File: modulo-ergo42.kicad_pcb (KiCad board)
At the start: 2 copper layers, 135.9 x 79.4 mm, 38 parts, among them J1 AudioJack4_Ground, J2 AudioJack4_Ground, J3 AudioJack4_Ground, J4 AudioJack4_Ground, SW1 SW_Push, SW10 SW_Push, SW11 SW_Push, SW12 SW_Push, SW13 SW_Push, SW14 SW_Push, SW15 SW_Push, SW16 SW_Push, SW17 SW_Push, SW18 SW_Push, SW19 SW_Push, SW2 SW_Push, SW20 SW_Push, SW21 SW_Push, SW22 SW_Push, SW23 SW_Push, SW24 SW_Push, SW25 SW_Push, SW26 SW_Push, SW27 SW_Push, SW28 SW_Push, SW29 SW_DIP_x02, SW3 SW_Push, SW4 SW_Push, SW5 SW_Push, SW6 SW_Push, SW7 SW_Push, SW8 SW_Push, SW9 SW_Push, U1 TCA9555PWR, U2 TCA9555PWR

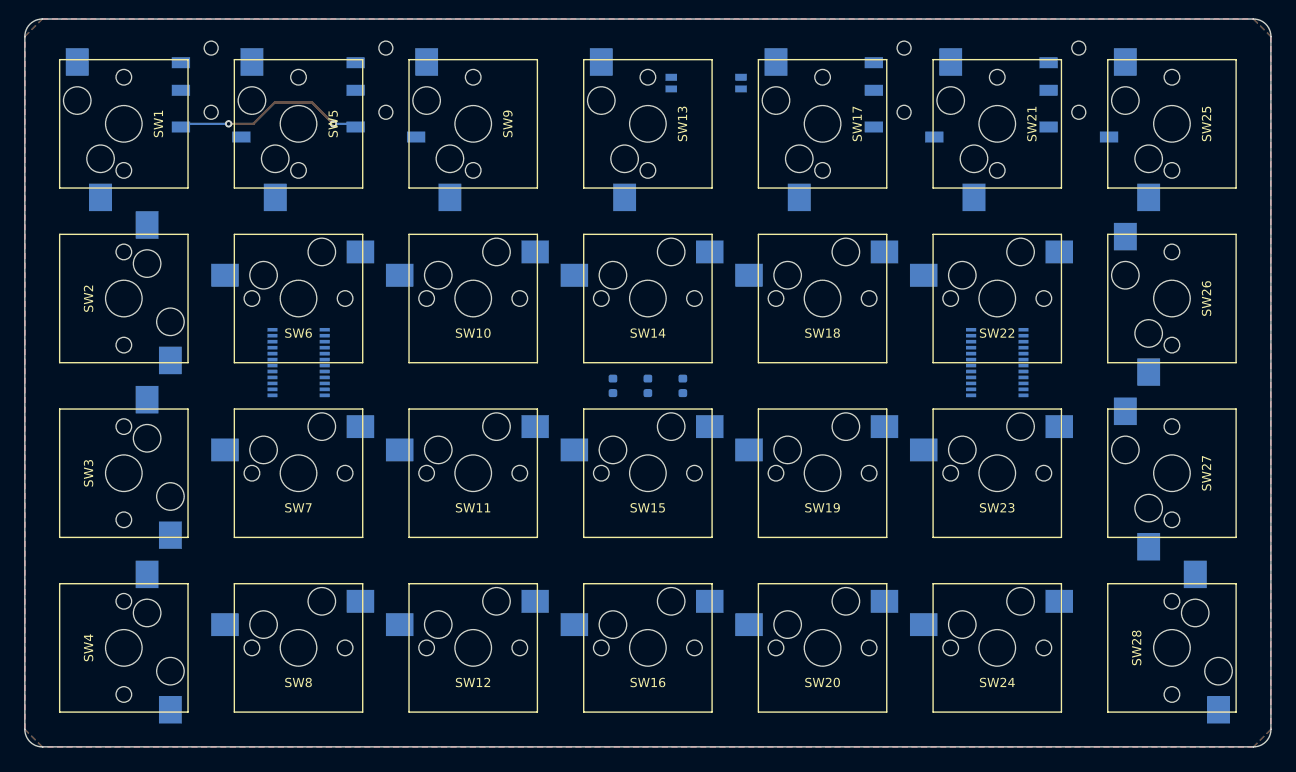
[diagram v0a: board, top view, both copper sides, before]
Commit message: Fix schematics
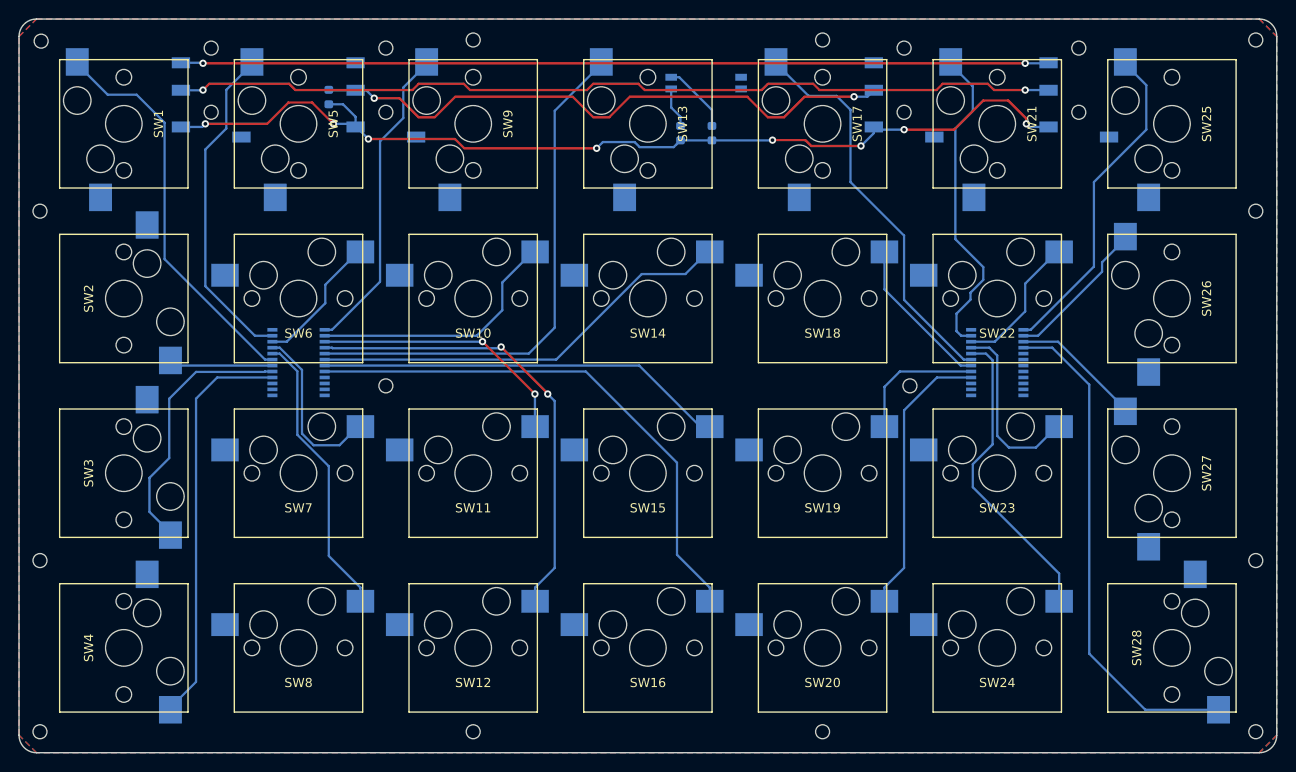
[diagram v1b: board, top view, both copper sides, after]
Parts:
- added ?: Screw_Hole, library:Screw_Hole, F.Cu at (56.9, 55.2)
- added ?: Screw_Hole, library:Screw_Hole, F.Cu at (142.2, 112.0)
- added ?: Screw_Hole, library:Screw_Hole, F.Cu at (189.5, 112.0)
- added ?: Screw_Hole, library:Screw_Hole, F.Cu at (189.5, 36.6)
- added ?: Screw_Hole, library:Screw_Hole, F.Cu at (94.6, 74.3)
- added ?: Screw_Hole, library:Screw_Hole, F.Cu at (151.8, 74.3)
- added ?: Screw_Hole, library:Screw_Hole, F.Cu at (56.9, 93.3)
- added ?: Screw_Hole, library:Screw_Hole, F.Cu at (189.5, 93.3)
- added ?: Screw_Hole, library:Screw_Hole, F.Cu at (189.5, 55.2)
- added ?: Screw_Hole, library:Screw_Hole, F.Cu at (142.2, 36.6)
- added ?: Screw_Hole, library:Screw_Hole, F.Cu at (104.1, 36.6)
- added ?: Screw_Hole, library:Screw_Hole, F.Cu at (57.0, 36.7)
- added ?: Screw_Hole, library:Screw_Hole, F.Cu at (56.9, 112.0)
- added ?: Screw_Hole, library:Screw_Hole, F.Cu at (104.1, 112.0)
- moved R1 44.2 mm to (88.4, 42.8), turned to 90 degrees
- moved R2 28.4 mm to (130.2, 46.7), turned to 90 degrees
- moved R3 27.6 mm to (126.7, 46.7), turned to 90 degrees
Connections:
- J1 pad R1: SDA1 -> SDA
- J1 pad R2: SCL1 -> SCL
- J2 pad R1: SDA2 -> SDA
- J2 pad R2: SCL2 -> SCL
- R1 pad 1: VCC -> 3V3
- R2 pad 1: VCC -> 3V3
- R3 pad 1: VCC -> 3V3
- U1 pad 22: SCL1 -> SCL
- U1 pad 23: SDA1 -> SDA
- U2 pad 21: VCC -> 3V3
- U2 pad 22: SCL2 -> SCL
- U2 pad 23: SDA2 -> SDA
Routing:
- net SDA: track 0.00 -> 97.5 mm, vias 0 -> 2
- net SCL: track 0.00 -> 94.7 mm, vias 0 -> 2
- net 3V3: track 21.3 -> 107.7 mm, vias 2 -> 8
- net INT: track 0.00 -> 65.6 mm, vias 0 -> 2
- net R4C4: track 0.00 -> 59.1 mm
- net R1C4: track 0.00 -> 57.3 mm
- net R4C7: track 0.00 -> 54.8 mm
- net R4C3: track 0.00 -> 50.4 mm, vias 0 -> 2
- net R2C4: track 0.00 -> 46.9 mm
- net R3C4: track 0.00 -> 44.8 mm
- net R4C1: track 0.00 -> 44.4 mm
- net R1C5: track 0.00 -> 43.8 mm
- net R1C1: track 0.00 -> 43.6 mm
- net R1C7: track 0.00 -> 36.2 mm
- net R1C2: track 0.00 -> 36.1 mm
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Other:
- board size 135.9 x 79.4 mm -> 137.2 x 80 mm
